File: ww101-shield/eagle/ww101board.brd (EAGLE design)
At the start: 59.1 x 64.6 mm, 58 parts

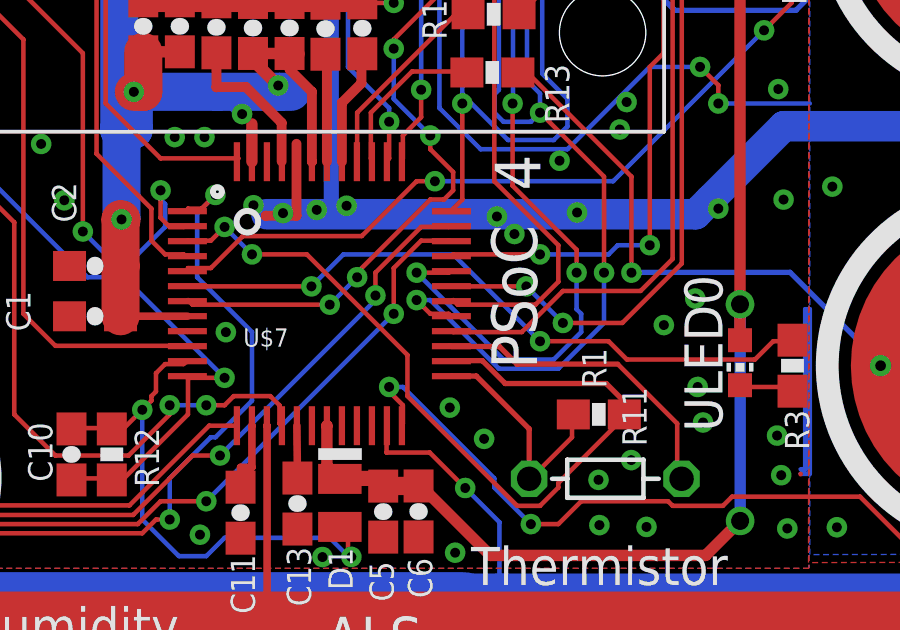
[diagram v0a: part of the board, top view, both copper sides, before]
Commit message: Updated Test Program
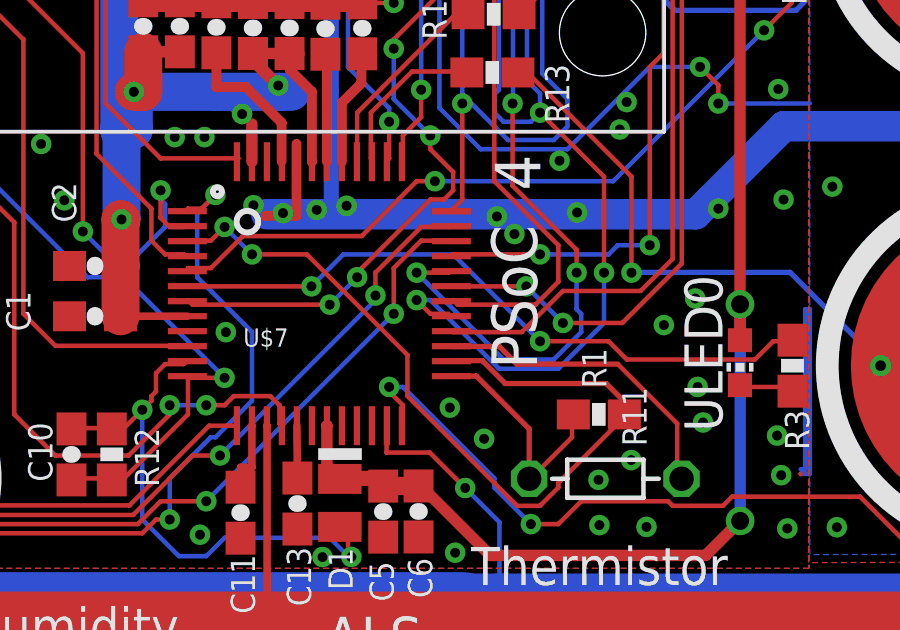
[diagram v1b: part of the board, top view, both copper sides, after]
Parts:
- moved MB0 9.60 mm to (24.7, 44.7)
- moved MB1 9.60 mm to (24.7, 54.3)
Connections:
- net MB0: now also JP1.2, R10.2, U$7.29; no longer JP1.1, R9.2, U$7.28
- net MB1: now also JP1.1, R9.2, U$7.28; no longer JP1.2, R10.2, U$7.29
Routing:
- net MB0: track 78.6 -> 76.2 mm, vias 5 -> 7
- net MB1: track 76.3 -> 78.6 mm, vias 7 -> 5
